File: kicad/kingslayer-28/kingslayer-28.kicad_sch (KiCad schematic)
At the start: 67 parts, among them IC1 STM32F303CCT7, K1 KEYSW, K10 KEYSW, K11 KEYSW, K12 KEYSW, K13 KEYSW, K14 KEYSW, K15 KEYSW, K16 KEYSW, K17 KEYSW, K18 KEYSW, K19 KEYSW, K2 KEYSW, K20 KEYSW, K21 KEYSW, K22 KEYSW, K23 KEYSW, K24 KEYSW, K25 KEYSW, K26 KEYSW, K27 KEYSW, K28 KEYSW, K3 KEYSW, K4 KEYSW, K5 KEYSW, K6 KEYSW, K7 KEYSW, K8 KEYSW, K9 KEYSW, Y1 FA-238_16.0000MB-C3

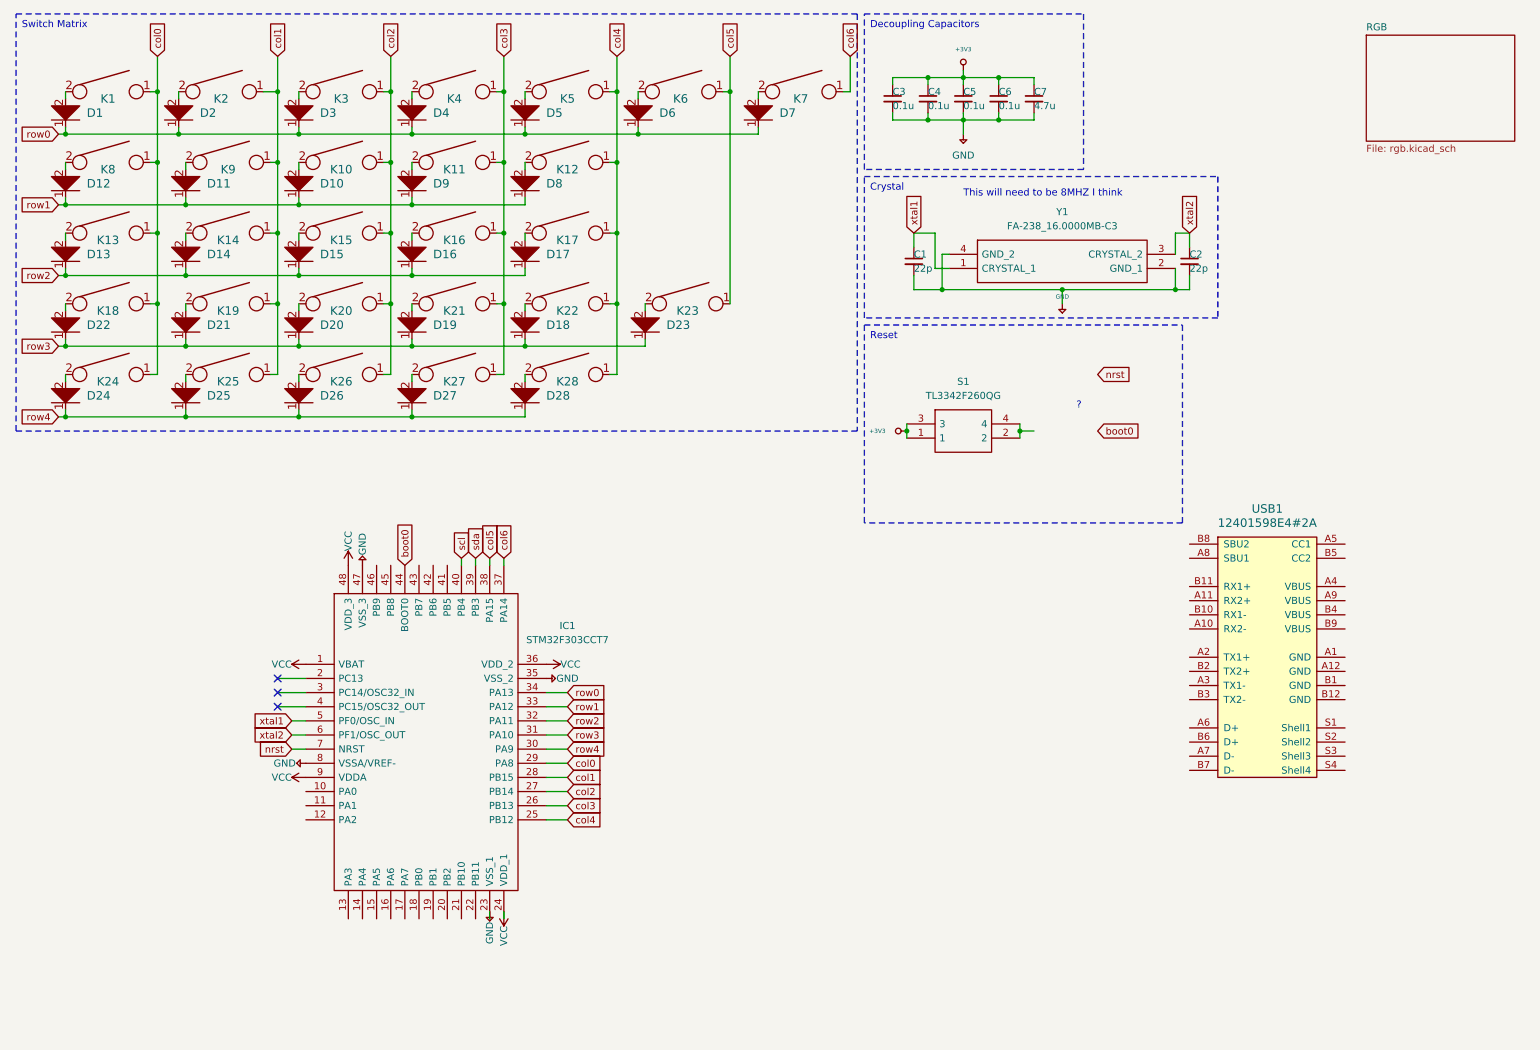
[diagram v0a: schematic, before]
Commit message: MCU done...
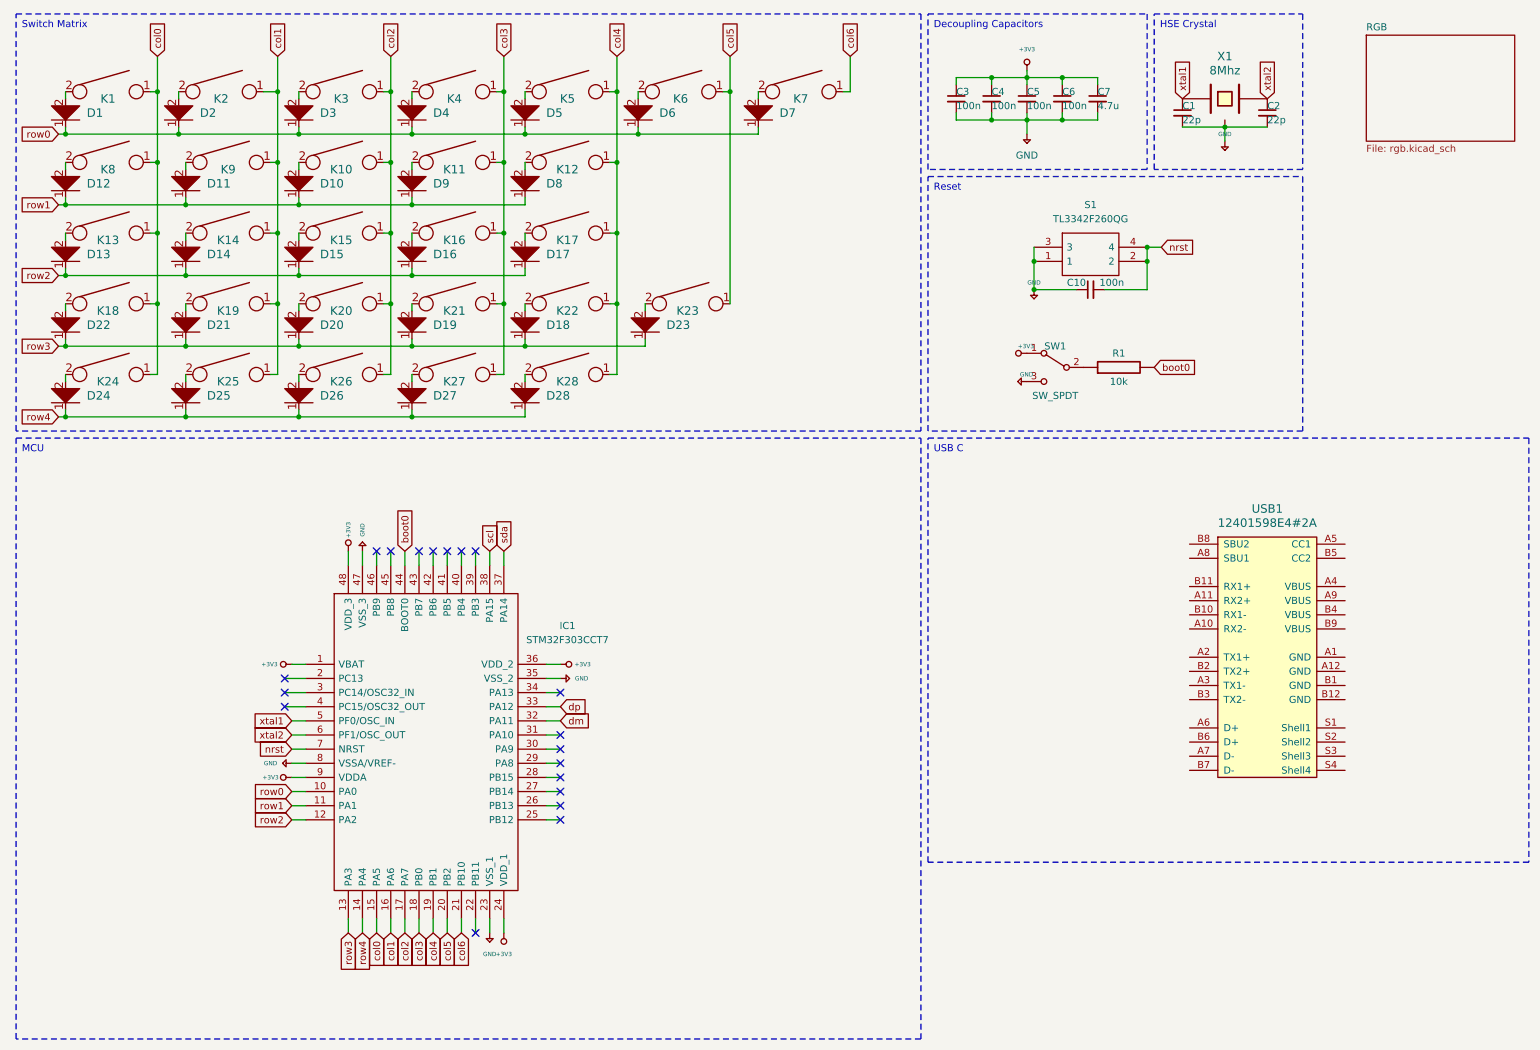
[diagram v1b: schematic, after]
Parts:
- removed Y1: FA-238_16.0000MB-C3, FA238160000MBC3, symbol FA-238_16.0000MB-C3:FA-238_16.0000MB-C3
- added C10: 100n, symbol Device:C_Small
- added R1: 10k, symbol keyboard_parts:R
- added SW1: SW_SPDT, symbol Switch:SW_SPDT
- added X1: 8Mhz, symbol keyboard_parts:XTAL_GND
- C3, C4, C5, C6: value 0.1u -> 100n
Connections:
- net VCC is gone; now on net +5V: IC1.1 (VBAT), IC1.24 (VDD_1), IC1.36 (VDD_2), IC1.48 (VDD_3), IC1.9 (VDDA)
- net +5V: now also C10.1, SW1.1 (A), SW1.3 (C), X1.3
- net boot0: now also R1.2
- net col0: now also IC1.15 (PA5); no longer IC1.29 (PA8)
- net col1: now also IC1.16 (PA6); no longer IC1.28 (PB15)
- net col2: now also IC1.17 (PA7); no longer IC1.27 (PB14)
- net col3: now also IC1.18 (PB0); no longer IC1.26 (PB13)
- net col4: now also IC1.19 (PB1); no longer IC1.25 (PB12)
- net col5: now also IC1.20 (PB2); no longer IC1.38 (PA15)
- net col6: now also IC1.21 (PB10); no longer IC1.37 (PA14)
- net nrst: now also S1.2, S1.4, C10.2
- net row0: now also IC1.10 (PA0); no longer IC1.34 (PA13)
- net row1: now also IC1.11 (PA1); no longer IC1.33 (PA12)
- net row2: now also IC1.12 (PA2); no longer IC1.32 (PA11)
- net row3: now also IC1.13 (PA3); no longer IC1.31 (PA10)
- net row4: now also IC1.14 (PA4); no longer IC1.30 (PA9)
- net scl: now also IC1.38 (PA15); no longer IC1.40 (PB4)
- net sda: now also IC1.37 (PA14); no longer IC1.39 (PB3)
- net xtal1: now also X1.1
- net xtal2: now also X1.2
- new net: R1.1, SW1.2 (B)
- new net dm: IC1.32 (PA11)
- new net dp: IC1.33 (PA12)
- no-connect marks 3 -> 19
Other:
- note removed: "?"
- note removed: "This will need to be 8MHZ I think"
- moved on the sheet: C1, C2, C3, C4, C5, C6, C7, S1
